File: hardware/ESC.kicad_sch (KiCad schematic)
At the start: 83 parts, among them J1 +, J2 -, J3 Conn_01x03, J4 +, J5 +, J6 +, J7 Conn_01x03, Q1 AGM60P30AP, Q2 AGM60P30AP, Q3 AGM60P30AP, Q4 AGM60P30AP, Q5 AGM60P30AP, Q6 AGM60P30AP, Q7 AGM60P30A, U1 DRV8323RSRGZR, U2 STM32G431CBTx, Y1 X322516MLB4SI

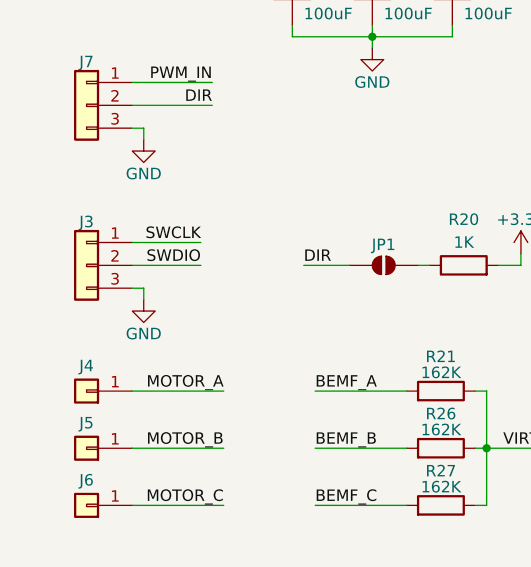
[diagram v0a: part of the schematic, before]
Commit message: started routing schematic
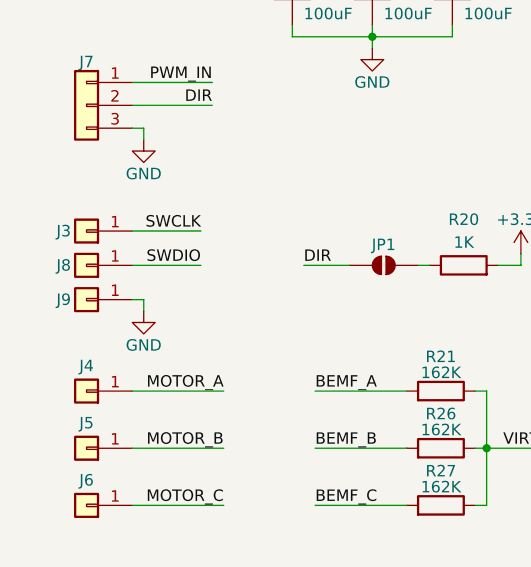
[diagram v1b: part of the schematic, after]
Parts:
- removed J3: Conn_01x03, Connector_PinHeader_2.54mm:PinHeader_1x03_P2.54mm_Vertical, symbol Connector_Generic:Conn_01x03
- added J3, J8, J9: +, Connector_Wire:SolderWirePad_1x01_SMD_2x4mm, symbol Connector_Generic:Conn_01x01
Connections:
- net GND: now also J9.1 (Pin_1)
- net SWCLK: now also J3.1 (Pin_1)
- net SWDIO: now also J8.1 (Pin_1)
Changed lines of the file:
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@@
 	(wire
 		(pts
-			(xy 29.21 92.71) (xy 29.21 91.44)
+			(xy 29.21 93.98) (xy 29.21 92.71)
 		)
 		(stroke
@@
 	(wire
 		(pts
-			(xy 27.94 86.36) (xy 35.56 86.36)
+			(xy 27.94 85.09) (xy 35.56 85.09)
 		)
 		(stroke
@@
 	(wire
 		(pts
-			(xy 29.21 91.44) (xy 27.94 91.44)
+			(xy 29.21 92.71) (xy 27.94 92.71)
 		)
 		(stroke
@@
 	)
 	(label "SWCLK"
-		(at 35.56 86.36 180)
+		(at 35.56 85.09 180)
 		(effects
 			(font
@@
 	)
 	(symbol
+		(lib_id "Connector_Generic:Conn_01x01")
+		(at 22.86 88.9 180)
+		(unit 1)
+		(exclude_from_sim no)
+		(in_bom yes)
+		(on_board yes)
+		(dnp no)
+		(property "Reference" "J8"
+			(at 20.32 88.9 0)
+			(effects
+				(font
+					(size 1.27 1.27)
+				)
+			)
+		)
+		(property "Value" "+"
+			(at 20.066 88.646 0)
+			(effects
+				(font
+					(size 2.54 2.54)
+				)
+				(hide yes)
+			)
+		)
+		(property "Footprint" "Connector_Wire:SolderWirePad_1x01_SMD_2x4mm"
+			(at 22.86 88.9 0)
+			(effects
+				(font
+					(size 1.27 1.27)
+				)
+				(hide yes)
+			)
+		)
+		(property "Datasheet" "~"
+			(at 22.86 88.9 0)
+			(effects
+				(font
+					(size 1.27 1.27)
+				)
+				(hide yes)
+			)
+		)
+		(property "Description" "Generic connector, single row, 01x01, script generated (kicad-library-utils/schlib/autogen/connector/)"
+			(at 22.86 88.9 0)
+			(effects
+				(font
+					(size 1.27 1.27)
+				)
+				(hide yes)
+			)
+		)
+		(pin "1"
+		)
+		(instances
+			(project "ESC"
+				(path "/4de1658d-a5e4-45f8-9b2f-349bf6ebe789"
+					(reference "J8")
+					(unit 1)
+				)
+			)
+		)
+	)
+	(symbol
 		(lib_id "Device:L")
 		(at 266.7 66.04 90)
@@
 	)
 	(symbol
-		(lib_id "Connector_Generic:Conn_01x03")
-		(at 22.86 88.9 0)
-		(mirror y)
-		(unit 1)
-		(exclude_from_sim no)
-		(in_bom yes)
-		(on_board yes)
-		(dnp no)
-		(property "Reference" "J3"
-			(at 22.86 84.074 0)
-			(effects
-				(font
-					(size 1.27 1.27)
-				)
-			)
-		)
-		(property "Value" "Conn_01x03"
-			(at 22.86 82.55 0)
-			(effects
-				(font
-					(size 1.27 1.27)
-				)
-				(hide yes)
-			)
-		)
-		(property "Footprint" "Connector_PinHeader_2.54mm:PinHeader_1x03_P2.54mm_Vertical"
-			(at 22.86 88.9 0)
-			(effects
-				(font
-					(size 1.27 1.27)
-				)
-				(hide yes)
-			)
-		)
-		(property "Datasheet" "~"
-			(at 22.86 88.9 0)
-			(effects
-				(font
-					(size 1.27 1.27)
-				)
-				(hide yes)
-			)
-		)
-		(property "Description" "Generic connector, single row, 01x03, script generated (kicad-library-utils/schlib/autogen/connector/)"
-			(at 22.86 88.9 0)
-			(effects
-				(font
-					(size 1.27 1.27)
-				)
-				(hide yes)
-			)
-		)
-		(pin "1"
-		)
-		(pin "2"
-		)
-		(pin "3"
-		)
-		(instances
-			(project "ESC"
-				(path "/4de1658d-a5e4-45f8-9b2f-349bf6ebe789"
-					(reference "J3")
-					(unit 1)
-				)
-			)
-		)
-	)
-	(symbol
 		(lib_id "Connector_Generic:Conn_01x01")
 		(at 22.86 102.87 180)
@@
 	(symbol
 		(lib_id "power:GND")
-		(at 29.21 92.71 0)
+		(at 29.21 93.98 0)
 		(unit 1)
 		(exclude_from_sim no)
@@
 		(dnp no)
 		(property "Reference" "#PWR047"
-			(at 29.21 99.06 0)
+			(at 29.21 100.33 0)
 			(effects
 				(font
@@
 		)
 		(property "Value" "GND"
-			(at 29.21 96.52 0)
+			(at 29.21 97.79 0)
 			(effects
 				(font
@@
 		)
 		(property "Footprint" ""
-			(at 29.21 92.71 0)
+			(at 29.21 93.98 0)
 			(effects
 				(font
@@
 		)
 		(property "Datasheet" ""
-			(at 29.21 92.71 0)
+			(at 29.21 93.98 0)
 			(effects
 				(font
@@
 		)
 		(property "Description" "Power symbol creates a global label with name \"GND\" , ground"
-			(at 29.21 92.71 0)
+			(at 29.21 93.98 0)
 			(effects
 				(font
@@
 	)
 	(symbol
+		(lib_id "Connector_Generic:Conn_01x01")
+		(at 22.86 92.71 180)
+		(unit 1)
+		(exclude_from_sim no)
+		(in_bom yes)
+		(on_board yes)
+		(dnp no)
+		(property "Reference" "J9"
+			(at 20.32 92.71 0)
+			(effects
+				(font
+					(size 1.27 1.27)
+				)
+			)
+		)
+		(property "Value" "+"
+			(at 20.066 92.456 0)
+			(effects
+				(font
+					(size 2.54 2.54)
+				)
+				(hide yes)
+			)
+		)
+		(property "Footprint" "Connector_Wire:SolderWirePad_1x01_SMD_2x4mm"
+			(at 22.86 92.71 0)
+			(effects
+				(font
+					(size 1.27 1.27)
+				)
+				(hide yes)
+			)
+		)
+		(property "Datasheet" "~"
+			(at 22.86 92.71 0)
+			(effects
+				(font
+					(size 1.27 1.27)
+				)
+				(hide yes)
+			)
+		)
+		(property "Description" "Generic connector, single row, 01x01, script generated (kicad-library-utils/schlib/autogen/connector/)"
+			(at 22.86 92.71 0)
+			(effects
+				(font
+					(size 1.27 1.27)
+				)
+				(hide yes)
+			)
+		)
+		(pin "1"
+		)
+		(instances
+			(project "ESC"
+				(path "/4de1658d-a5e4-45f8-9b2f-349bf6ebe789"
+					(reference "J9")
+					(unit 1)
+				)
+			)
+		)
+	)
+	(symbol
 		(lib_id "power:+3.3VA")
 		(at 187.96 29.21 0)
@@
 					(unit 1)
 				)
+			)
+		)
+	)
+	(symbol
+		(lib_id "Connector_Generic:Conn_01x01")
+		(at 22.86 85.09 180)
+		(unit 1)
+		(exclude_from_sim no)
+		(in_bom yes)
+		(on_board yes)
+		(dnp no)
+		(property "Reference" "J3"
+			(at 20.32 85.09 0)
+			(effects
+				(font
+					(size 1.27 1.27)
+				)
+			)
+		)
+		(property "Value" "+"
+			(at 20.066 84.836 0)
+			(effects
+				(font
+					(size 2.54 2.54)
+				)
+				(hide yes)
+			)
+		)
+		(property "Footprint" "Connector_Wire:SolderWirePad_1x01_SMD_2x4mm"
+			(at 22.86 85.09 0)
+			(effects
+				(font
+					(size 1.27 1.27)
+				)
+				(hide yes)
+			)
+		)
+		(property "Datasheet" "~"
+			(at 22.86 85.09 0)
+			(effects
+				(font
+					(size 1.27 1.27)
+				)
+				(hide yes)
+			)
+		)
+		(property "Description" "Generic connector, single row, 01x01, script generated (kicad-library-utils/schlib/autogen/connector/)"
+			(at 22.86 85.09 0)
+			(effects
+				(font
+					(size 1.27 1.27)
+				)
+				(hide yes)
+			)
+		)
+		(pin "1"
+		)
+		(instances
+			(project "ESC"
+				(path "/4de1658d-a5e4-45f8-9b2f-349bf6ebe789"
+					(reference "J3")
+					(unit 1)
+				)
